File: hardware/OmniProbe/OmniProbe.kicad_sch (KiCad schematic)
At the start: 62 parts, among them J1 USB_C_Receptacle_USB2.0_16P, J10 Conn_01x04_Socket, J2 Conn_ARM_JTAG_SWD_10, J6 Conn_01x03_Socket, J7 Conn_01x03_Socket, J8 Conn_01x16_Socket, J9 Conn_01x04_Socket, U1 RP2040, U2 W25Q128JVP, U3 AP2112K-3.3, U4 TXS0108EPW, U5 TPD2E2U06DCK, Y1 12MHz

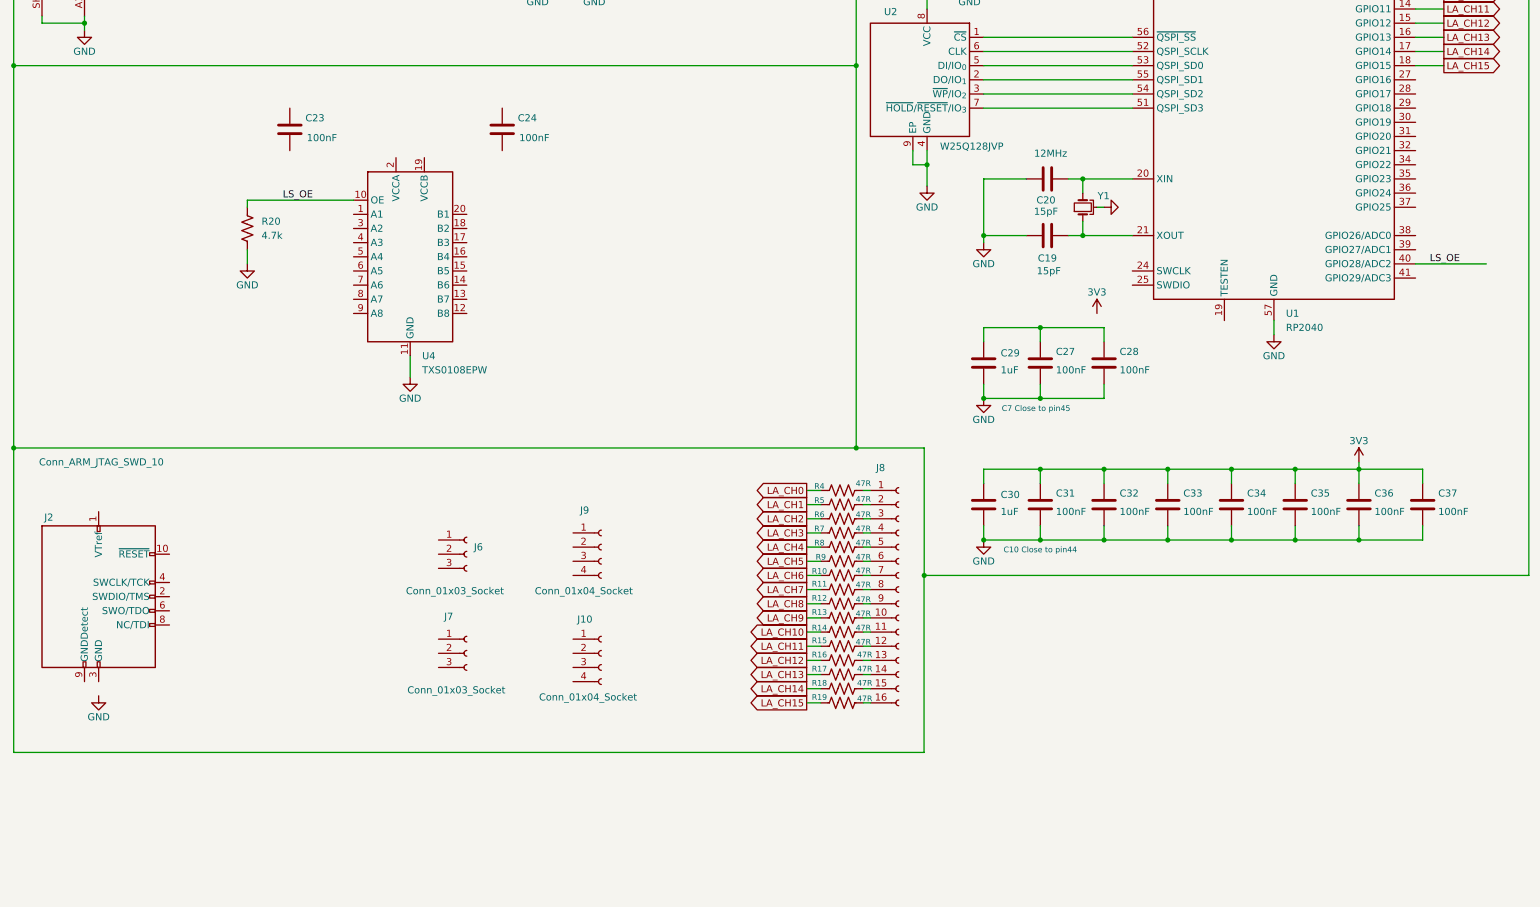
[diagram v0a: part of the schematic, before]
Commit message: V0
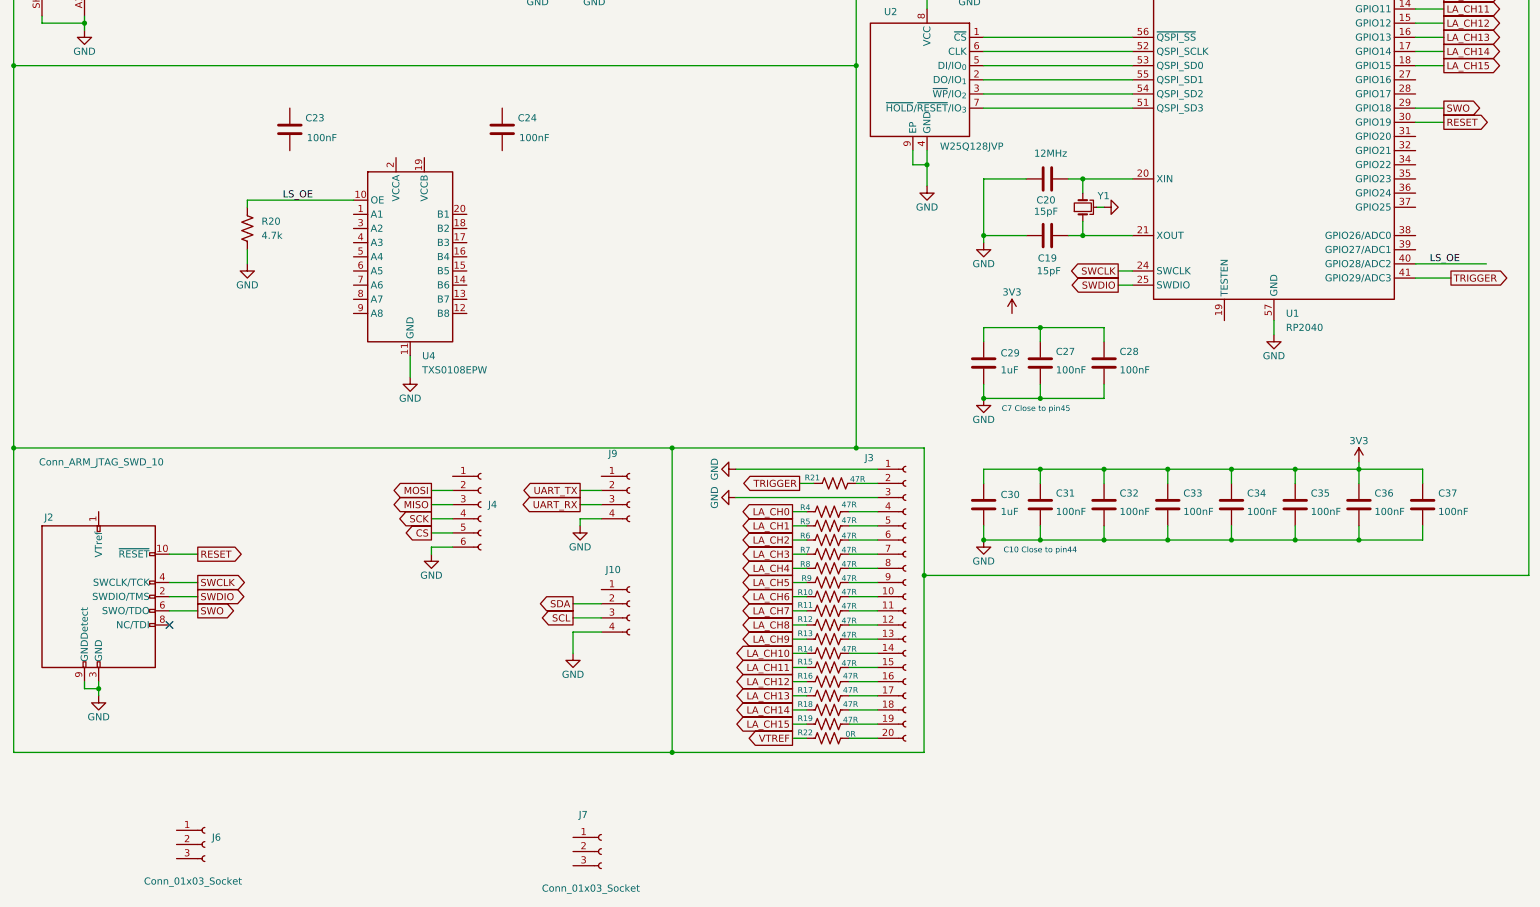
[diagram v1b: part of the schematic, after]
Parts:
- removed J8: Conn_01x16_Socket, Connector_PinHeader_2.54mm:PinHeader_1x16_P2.54mm_Vertical, symbol Connector:Conn_01x16_Socket
- added J3: Conn_01x20_Socket, Connector_PinHeader_2.54mm:PinHeader_1x20_P2.54mm_Vertical, symbol Connector:Conn_01x20_Socket
- added J4: Conn_01x06_Socket, Connector_PinHeader_2.54mm:PinHeader_1x06_P2.54mm_Vertical, symbol Connector:Conn_01x06_Socket
- added R21: 47R, Resistor_SMD:R_0603_1608Metric, symbol Device:R_US
- added R22: 0R, Resistor_SMD:R_0603_1608Metric, symbol Device:R_US
- C19, C20: footprint Capacitor_SMD:C_0603_1608Metric -> Capacitor_SMD:C_0402_1005Metric
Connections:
- net GND: now also J10.4 (Pin_4), J2.3 (GND), J2.5 (GND), J2.9 (GNDDetect), J9.4 (Pin_4), J3.1 (Pin_1), J3.3 (Pin_3), J4.6 (Pin_6)
- net SDA: now reaches J10.2 (Pin_2)
- net SCL: now reaches J10.3 (Pin_3)
- net at R16.2: now also J3.16 (Pin_16)
- net at R13.2: now also J3.13 (Pin_13)
- net RESET: now reaches J2.10 (~{RESET})
- net RESET: now also U1.30 (GPIO19)
- net SWDIO: now reaches J2.2 (SWDIO/TMS)
- net SWDIO: now also U1.25 (SWDIO)
- net SWCLK: now reaches J2.4 (SWCLK/TCK)
- net SWCLK: now also U1.24 (SWCLK)
- net SWO: now reaches J2.6 (SWO/TDO)
- net SWO: now also U1.29 (GPIO18)
- net UART_TX: now reaches J9.2 (Pin_2)
- net UART_RX: now reaches J9.3 (Pin_3)
- net at R14.2: now also J3.14 (Pin_14)
- net at R10.2: now also J3.10 (Pin_10)
- net at R8.2: now also J3.8 (Pin_8)
- net at R7.2: now also J3.7 (Pin_7)
- net at R15.2: now also J3.15 (Pin_15)
- net at R6.2: now also J3.6 (Pin_6)
- net at R18.2: now also J3.18 (Pin_18)
- net at R4.2: now also J3.4 (Pin_4)
- net at R17.2: now also J3.17 (Pin_17)
- net at R19.2: now also J3.19 (Pin_19)
- net at R5.2: now also J3.5 (Pin_5)
- net at R9.2: now also J3.9 (Pin_9)
- net at R11.2: now also J3.11 (Pin_11)
- net at R12.2: now also J3.12 (Pin_12)
- net TRIGGER: now reaches U1.41 (GPIO29/ADC3)
- net TRIGGER: now also R21.1
- new net: J3.2 (Pin_2), R21.2
- new net: J3.20 (Pin_20), R22.2
- new net CS: J4.5 (Pin_5)
- new net MISO: J4.3 (Pin_3)
- new net MOSI: J4.2 (Pin_2)
- new net SCK: J4.4 (Pin_4)
- new net VTREF: R22.1
- no-connect marks 2 -> 3
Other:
- moved on the sheet: J10, J6, J7, J9, R10, R11, R12, R13, R14, R15, R16, R17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

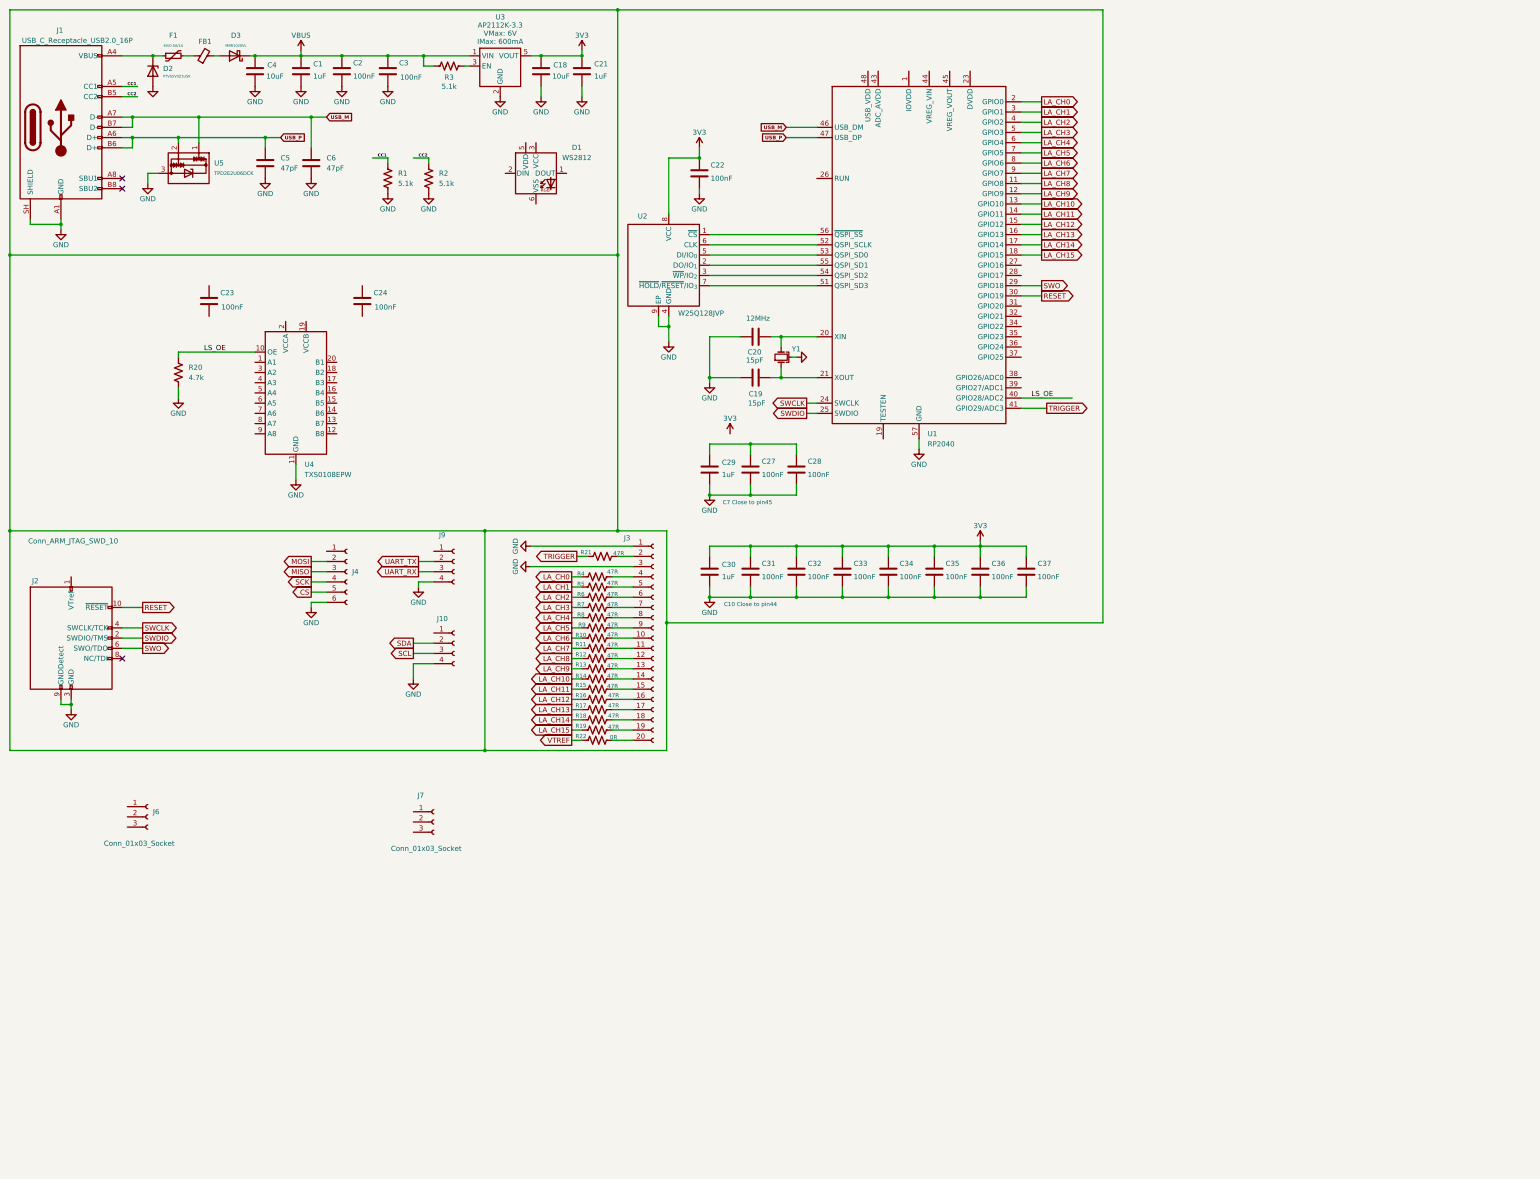
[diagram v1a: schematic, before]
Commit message: v0.1
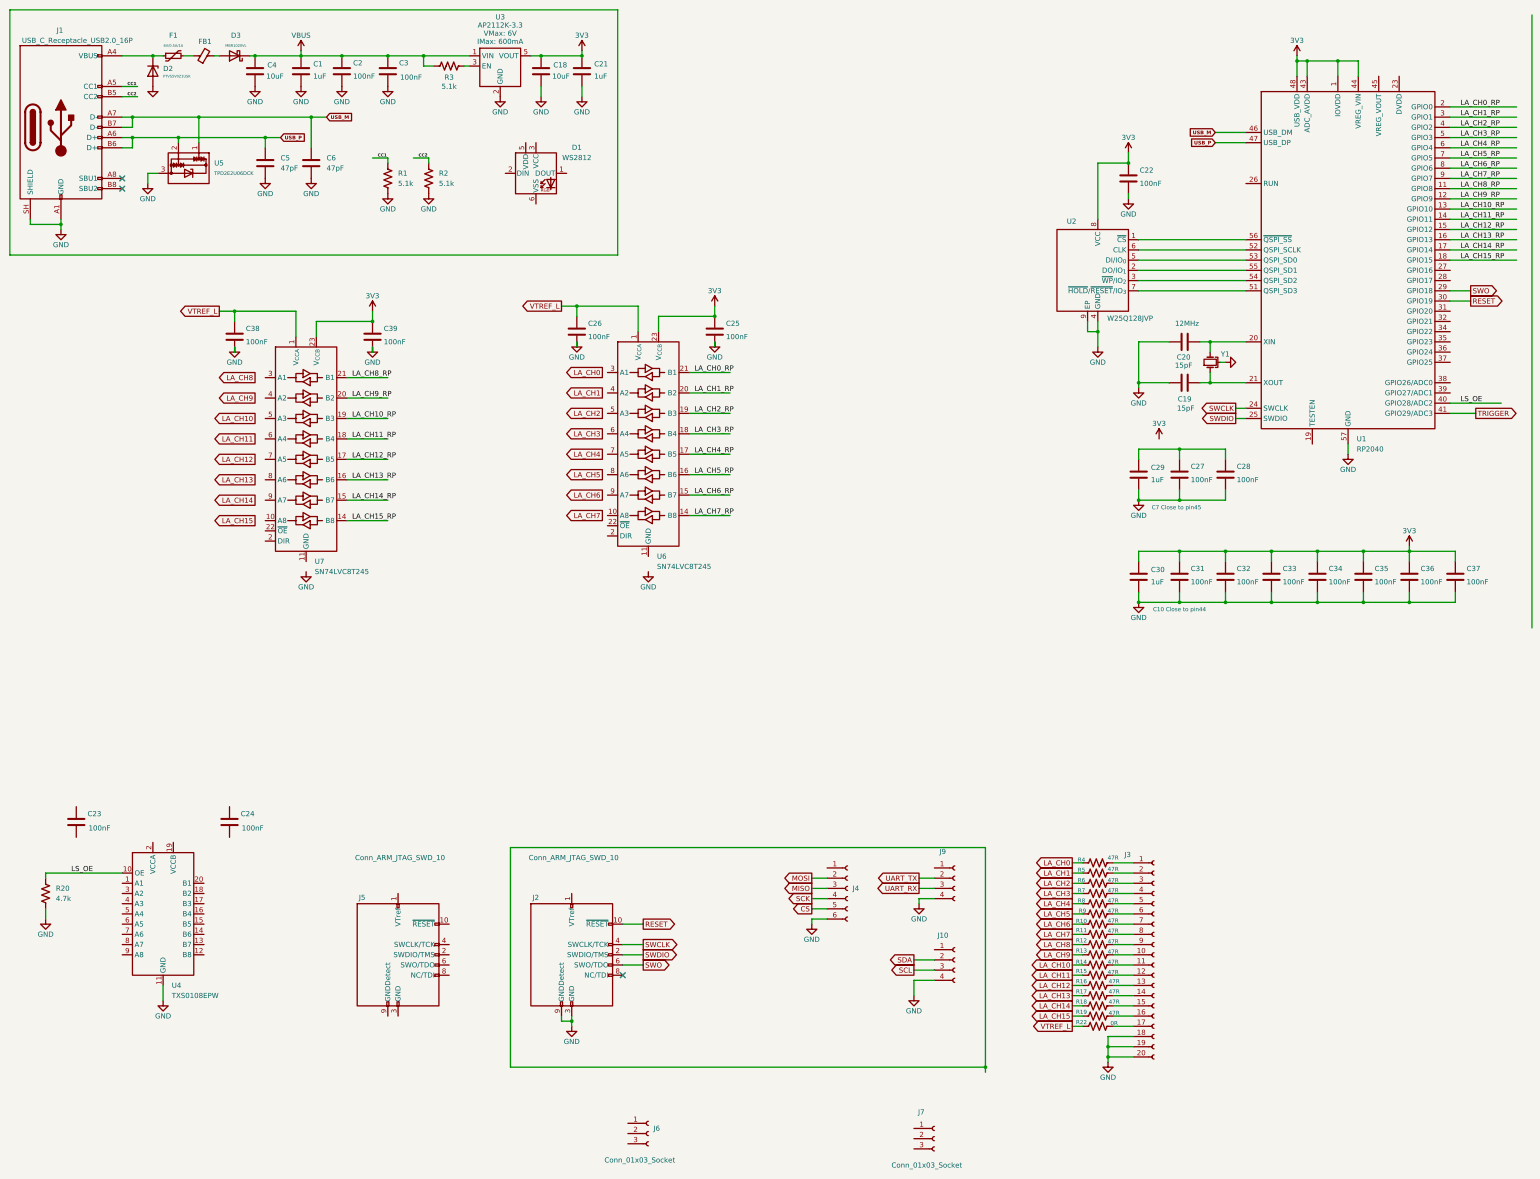
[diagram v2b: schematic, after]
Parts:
- removed R21: 47R, Resistor_SMD:R_0603_1608Metric, symbol Device:R_US
- added C25, C26, C38, C39: 100nF, Capacitor_SMD:C_0603_1608Metric, symbol Device:C
- added J5: Conn_ARM_JTAG_SWD_10, Connector_PinHeader_1.27mm:PinHeader_2x05_P1.27mm_Vertical, symbol Connector:Conn_ARM_JTAG_SWD_10
- added U6, U7: SN74LVC8T245, Package_SO:TSSOP-24_4.4x7.8mm_P0.65mm, symbol Logic_LevelTranslator:SN74LVC8T245
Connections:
- net 3V3: now also U1.1 (IOVDD), U1.10 (IOVDD), U1.22 (IOVDD), U1.33 (IOVDD), U1.42 (IOVDD), U1.43 (ADC_AVDD), U1.44 (VREG_VIN), U1.48 (USB_VDD), U1.49 (IOVDD), C25.1, C39.1, U6.23 (V_{CCB}), U6.24 (V_{CCB}), U7.23 (V_{CCB}), U7.24 (V_{CCB})
- net GND: now also J3.18 (Pin_18), J3.19 (Pin_19), J3.20 (Pin_20), C25.2, C26.2, C38.2, C39.2; no longer J3.1 (Pin_1), J3.3 (Pin_3)
- net LA_CH0: no longer U1.2 (GPIO0)
- net LA_CH1: no longer U1.3 (GPIO1)
- net LA_CH10: no longer U1.13 (GPIO10)
- net LA_CH11: no longer U1.14 (GPIO11)
- net LA_CH12: no longer U1.15 (GPIO12)
- net LA_CH13: no longer U1.16 (GPIO13)
- net LA_CH14: no longer U1.17 (GPIO14)
- net LA_CH15: no longer U1.18 (GPIO15)
- net LA_CH2: no longer U1.4 (GPIO2)
- net LA_CH3: no longer U1.5 (GPIO3)
- net LA_CH4: no longer U1.6 (GPIO4)
- net LA_CH5: no longer U1.7 (GPIO5)
- net LA_CH6: no longer U1.8 (GPIO6)
- net LA_CH7: no longer U1.9 (GPIO7)
- net LA_CH8: no longer U1.11 (GPIO8)
- net LA_CH9: no longer U1.12 (GPIO9)
- net at R16.2: now also J3.13 (Pin_13); no longer J3.16 (Pin_16)
- net at R13.2: now also J3.10 (Pin_10); no longer J3.13 (Pin_13)
- net at R14.2: now also J3.11 (Pin_11); no longer J3.14 (Pin_14)
- net at R10.2: now also J3.7 (Pin_7); no longer J3.10 (Pin_10)
- net at R11.2: now also J3.8 (Pin_8); no longer J3.11 (Pin_11)
- net at J3.12 (Pin_12): now also R15.2; no longer R12.2
- net at J3.15 (Pin_15): now also R18.2; no longer R15.2
- net at R17.2: now also J3.14 (Pin_14); no longer J3.17 (Pin_17)
- net at R19.2: now also J3.16 (Pin_16); no longer J3.19 (Pin_19)
- net at J3.2 (Pin_2): now also R5.2
- net at R22.2: now also J3.17 (Pin_17); no longer J3.20 (Pin_20)
- net at R4.2: now also J3.1 (Pin_1); no longer J3.4 (Pin_4)
- net at J3.5 (Pin_5): now also R8.2; no longer R5.2
- net at R6.2: now also J3.3 (Pin_3); no longer J3.6 (Pin_6)
- net at R7.2: now also J3.4 (Pin_4); no longer J3.7 (Pin_7)
- net at R9.2: now also J3.6 (Pin_6); no longer J3.9 (Pin_9)
- net VTREF renamed VTREF_L
- net VTREF_L: now also C26.1, C38.1, U6.1 (V_{CCA}), U7.1 (V_{CCA})
- new net: U7.11 (GND), U7.12 (GND), U7.13 (GND)
- new net: J5.3 (GND), J5.5 (GND)
- new net: J3.9 (Pin_9), R12.2
- new net: U6.11 (GND), U6.12 (GND), U6.13 (GND)
- new net LA_CH0_RP: U1.2 (GPIO0), U6.21 (B1)
- new net LA_CH10_RP: U1.13 (GPIO10), U7.19 (B3)
- new net LA_CH11_RP: U1.14 (GPIO11), U7.18 (B4)
- new net LA_CH12_RP: U1.15 (GPIO12), U7.17 (B5)
- new net LA_CH13_RP: U1.16 (GPIO13), U7.16 (B6)
- new net LA_CH14_RP: U1.17 (GPIO14), U7.15 (B7)
- new net LA_CH15_RP: U1.18 (GPIO15), U7.14 (B8)
- new net LA_CH1_RP: U1.3 (GPIO1), U6.20 (B2)
- new net LA_CH2_RP: U1.4 (GPIO2), U6.19 (B3)
- new net LA_CH3_RP: U1.5 (GPIO3), U6.18 (B4)
- new net LA_CH4_RP: U1.6 (GPIO4), U6.17 (B5)
- new net LA_CH5_RP: U1.7 (GPIO5), U6.16 (B6)
- new net LA_CH6_RP: U1.8 (GPIO6), U6.15 (B7)
- new net LA_CH7_RP: U1.9 (GPIO7), U6.14 (B8)
- new net LA_CH8_RP: U1.11 (GPIO8), U7.21 (B1)
- new net LA_CH9_RP: U1.12 (GPIO9), U7.20 (B2)
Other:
- moved on the sheet: C19, C20, C22, C23, C24, C27, C28, C29, C30, C31, C32, C33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
